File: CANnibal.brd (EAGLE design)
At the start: 15.2 x 36.2 mm, 22 parts, among them J1 POGOPIN-CONN-4, J3 455-1750-1-ND, J6 455-1750-1-ND, U1 STM32F042C6T6, U2 MF-REG-SOT235-3.3V-300mA

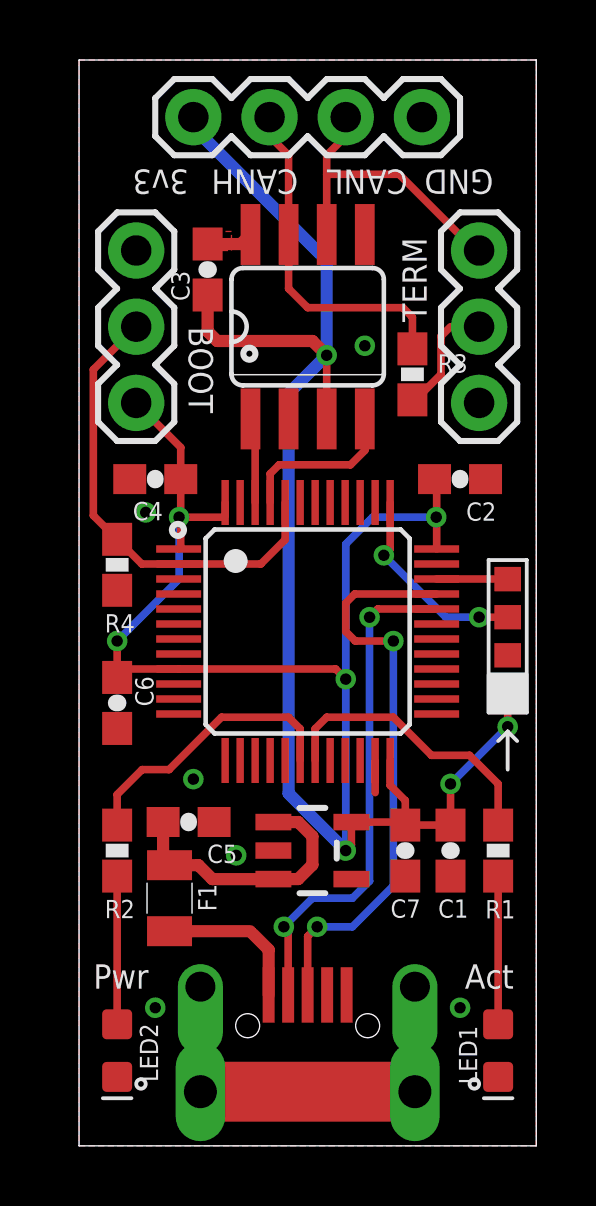
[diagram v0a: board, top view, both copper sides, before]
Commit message: Cleanup
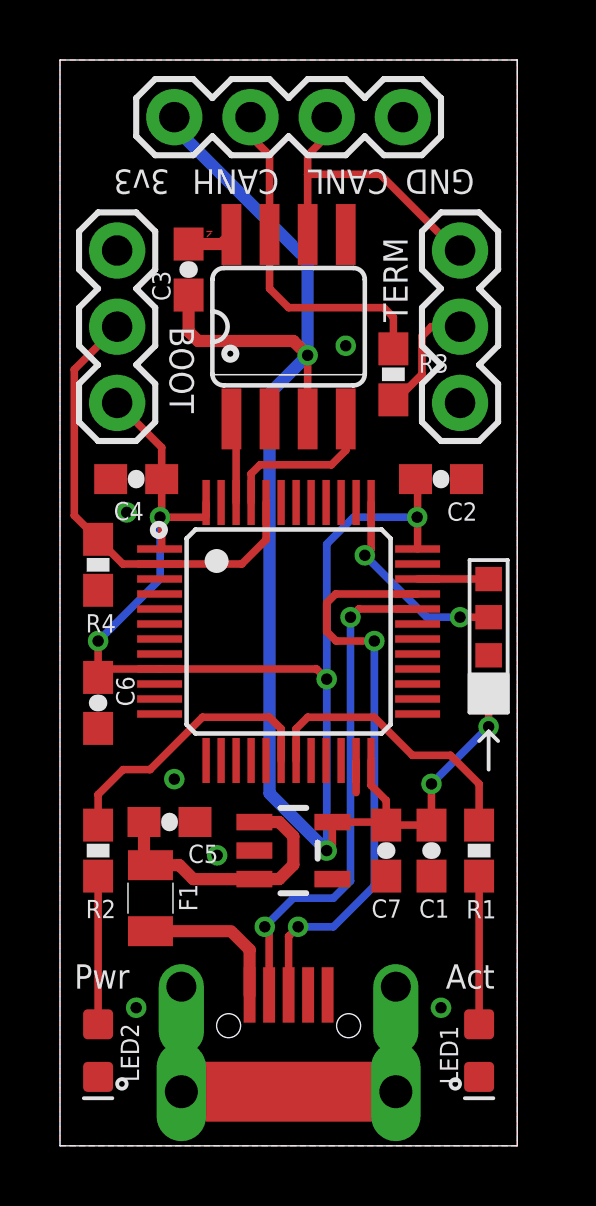
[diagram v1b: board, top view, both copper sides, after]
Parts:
- moved C2 0.64 mm to (12.7, 22.2)
- moved DA1 0.64 mm to (7.62, 27.3)
- moved U$4 0.64 mm to (7.62, 1.91)
- moved U1 0.64 mm to (7.62, 17.1)
- moved U2 0.64 mm to (7.78, 9.84)
- moved F1 0.64 mm to (3.02, 8.26)
- moved J2 0.64 mm to (3.81, 34.3)
- moved C6 0.64 mm to (1.27, 14.8)
- moved J3 0.64 mm to (1.91, 24.8)
- moved LED2 0.64 mm to (1.27, 3.17)
- moved R2 0.64 mm to (1.27, 9.84)
- moved R4 0.64 mm to (1.27, 19.4)
- moved C1 0.63 mm to (12.4, 9.84)
- moved C3 0.63 mm to (4.29, 29.2)
- moved C4 0.63 mm to (2.54, 22.2)
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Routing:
- net N$3: track 3.02 -> 3.98 mm
